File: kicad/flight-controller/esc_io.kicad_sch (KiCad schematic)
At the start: 10 parts, among them J19 ESC2, J20 FC UBEC Input, J22 ESC1, Q1 reverse polarity protection, Q2 reverse polarity protection

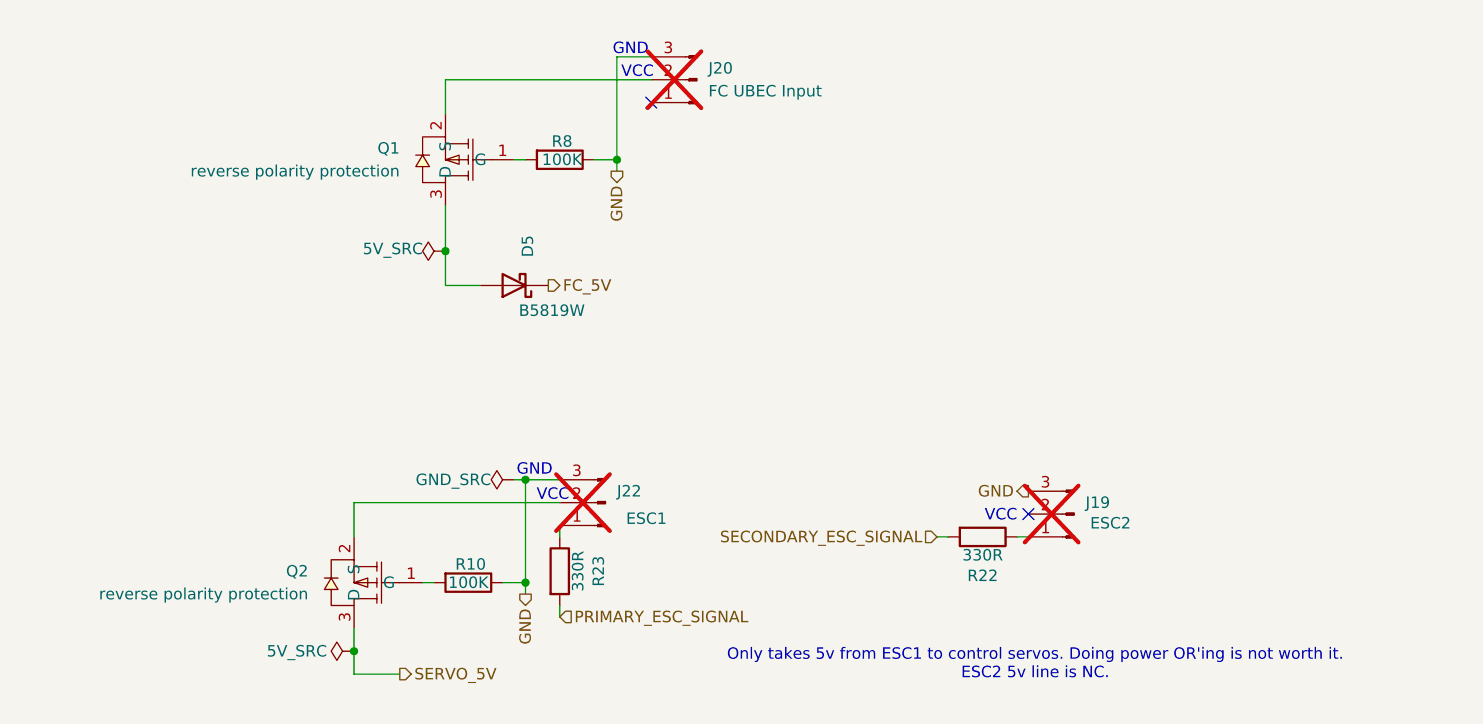
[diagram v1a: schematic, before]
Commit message: Kicad FC v3.1 complete, Mission Controller and UWB boards v1 complete, firmware v2 complete!
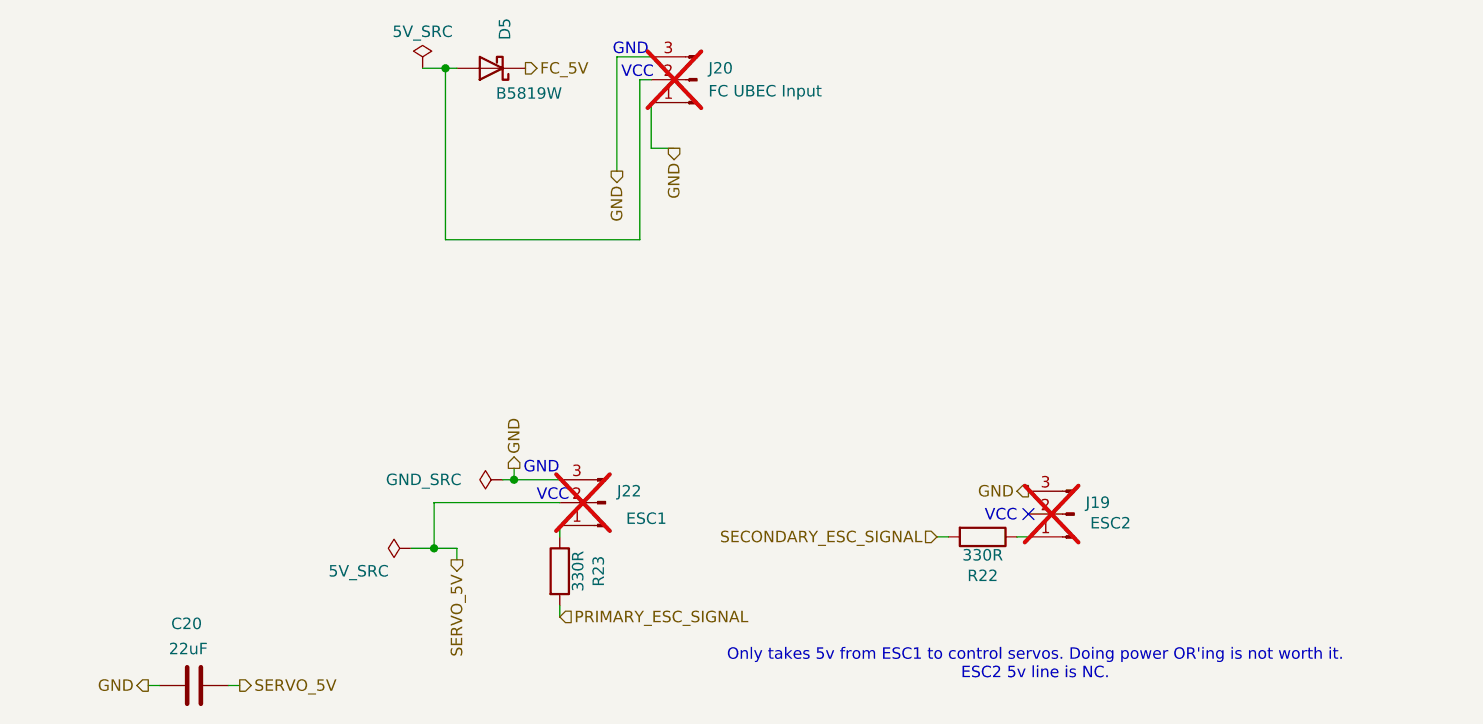
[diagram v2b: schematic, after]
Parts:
- removed Q1, Q2: reverse polarity protection, easyeda2kicad:SOT-23-3_L2.9-W1.6-P1.90-LS2.8-BR, symbol easyeda2kicad:AO3407A
- removed R10, R8: 100K, Resistor_SMD:R_0402_1005Metric, symbol Device:R
- added C20: 22uF, Capacitor_SMD:C_0805_2012Metric, symbol Device:C
- D5: Notes ESC1 UBEC diode -> FC UBEC input diode (J20 -> FC_5V)
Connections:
- net GND: now also J20.1 (Pin_1), C20.2
- net SERVO_5V: now also J22.2 (Pin_2), C20.1
- net at J20.2 (Pin_2): now also D5.2 (A)
- no-connect marks 2 -> 1
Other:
- moved on the sheet: D5
